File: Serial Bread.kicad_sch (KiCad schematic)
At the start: 20 parts, among them J1 TYPE-C-31-M-12, J2 Conn_02x04_Top_Bottom, U1 CH340C, U2 AP2112K-3.3

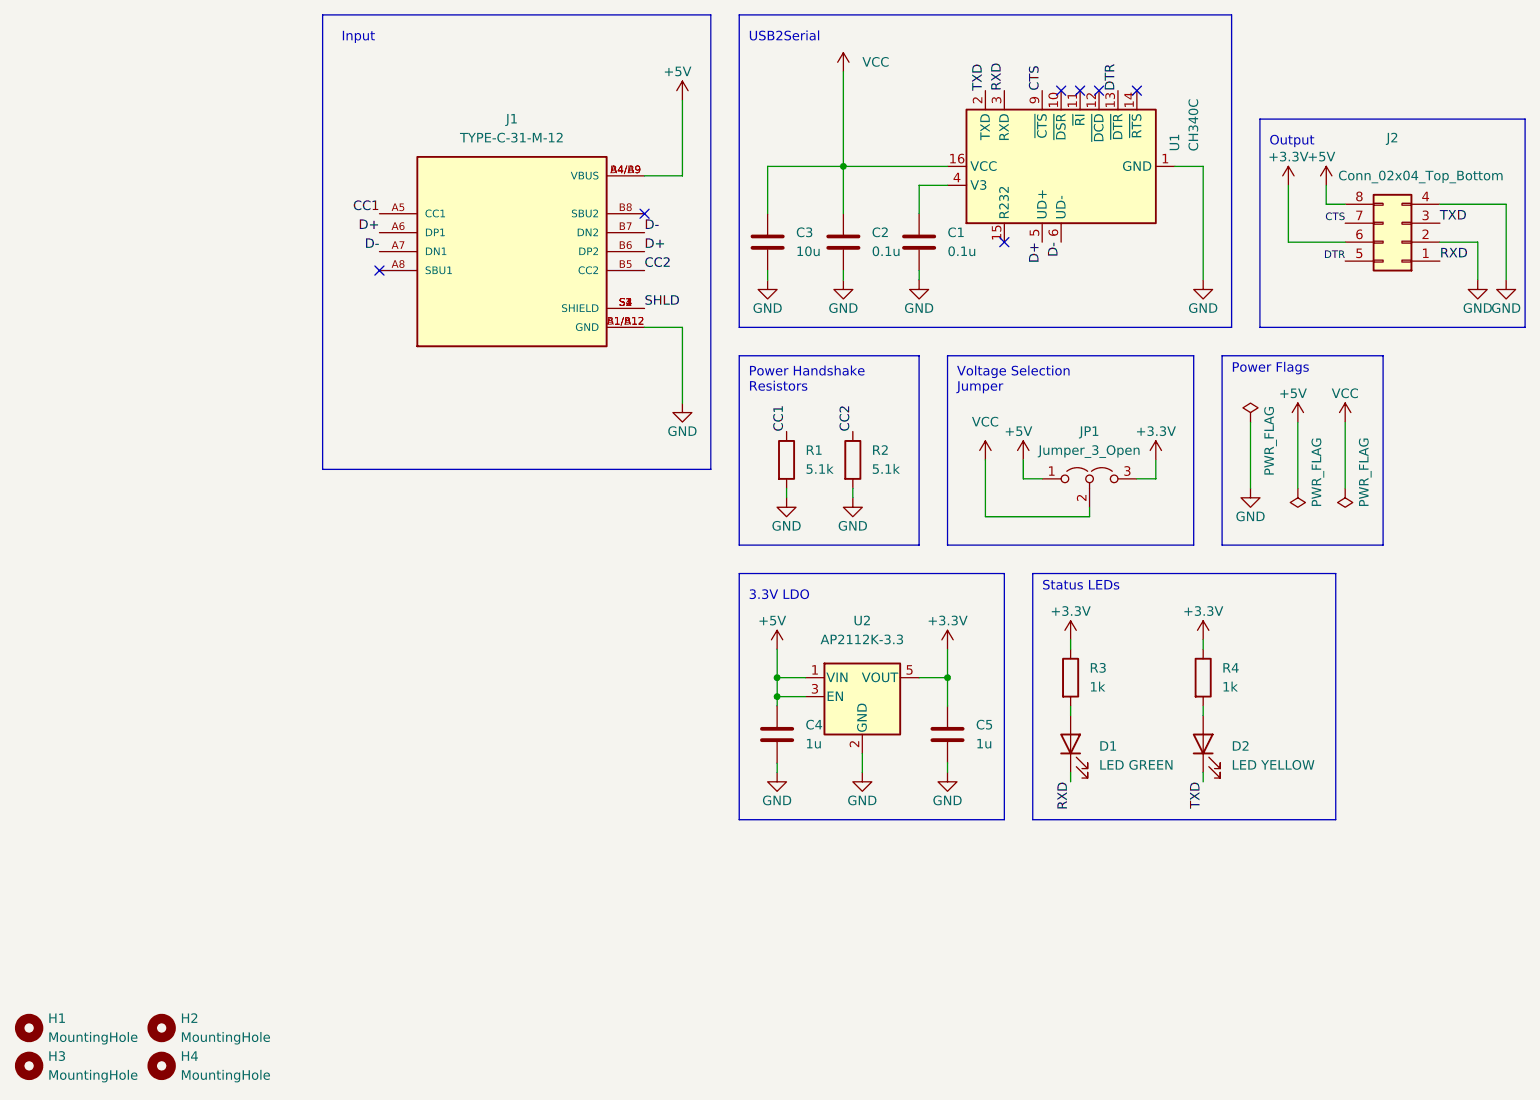
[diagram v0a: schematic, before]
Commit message: Initial commit R1.1
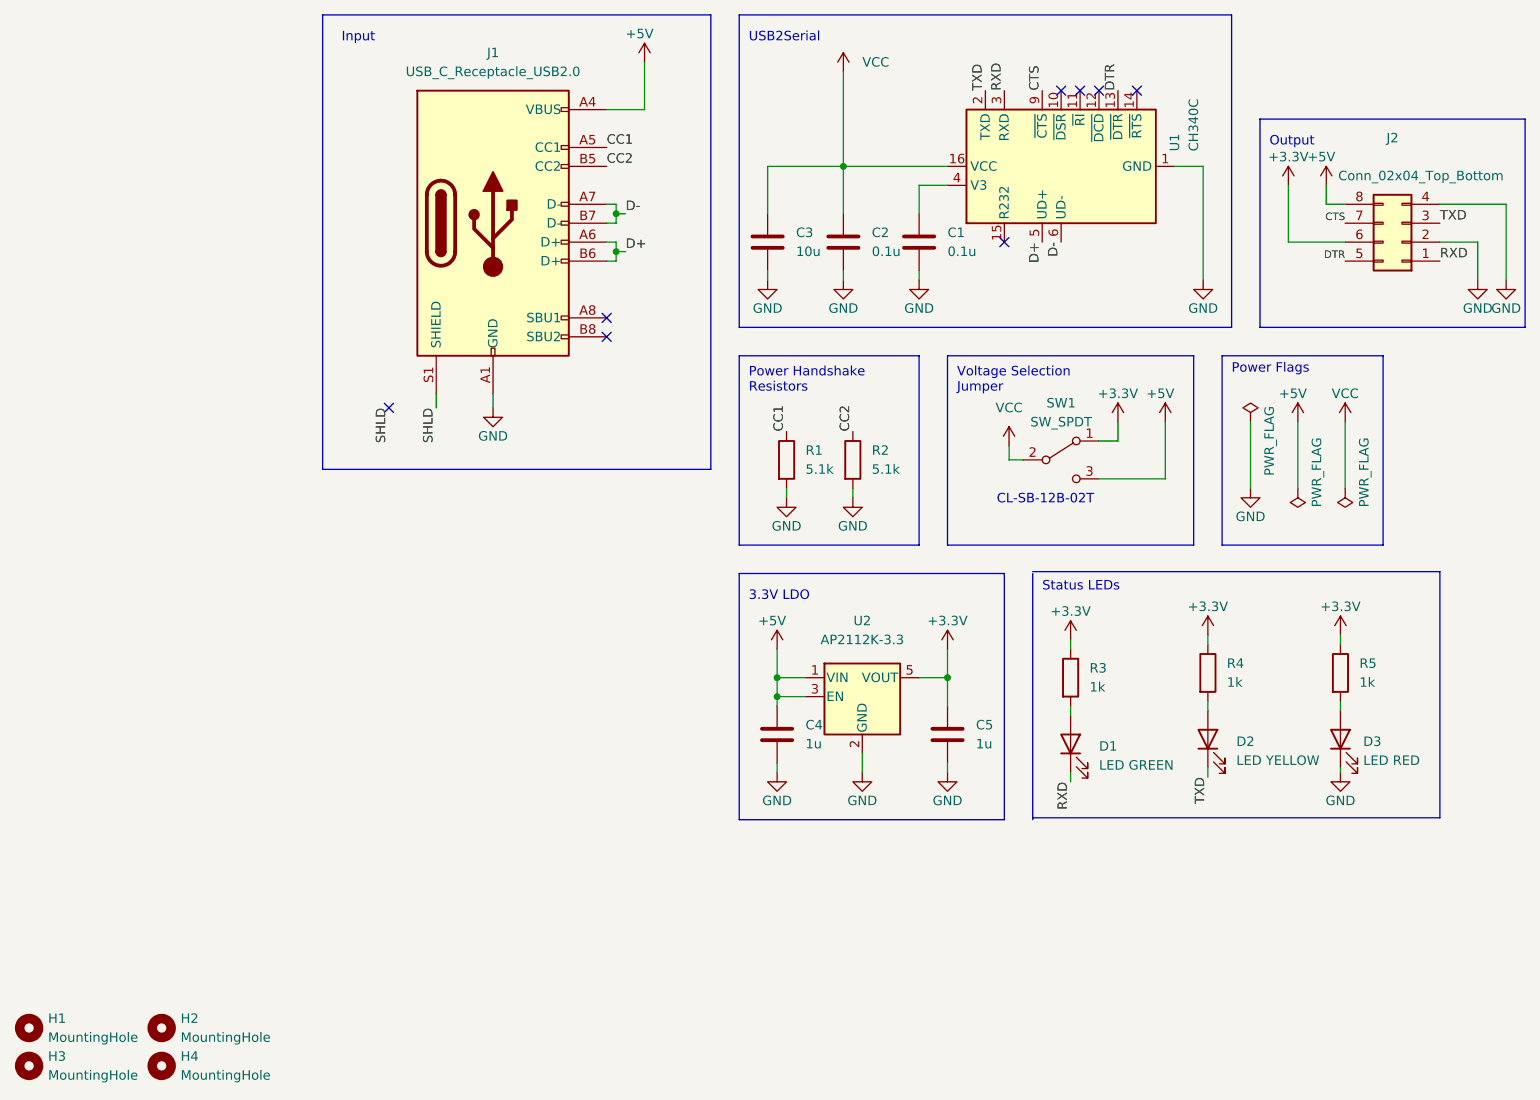
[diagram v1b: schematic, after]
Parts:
- removed J1: TYPE-C-31-M-12, SnapEDA Library:HRO_TYPE-C-31-M-12, symbol TYPE-C-31-M-12:TYPE-C-31-M-12
- removed JP1: Jumper_3_Open, Connector_PinHeader_1.27mm:PinHeader_1x03_P1.27mm_Vertical, symbol Jumper:Jumper_3_Open
- added D3: LED RED, LED_SMD:LED_0603_1608Metric, symbol Device:LED
- added J1: USB_C_Receptacle_USB2.0, Connector_USB:USB_C_Receptacle_HRO_TYPE-C-31-M-12, symbol Connector:USB_C_Receptacle_USB2.0
- added R5: 1k, Resistor_SMD:R_0402_1005Metric, symbol Device:R
- added SW1: SW_SPDT, Custom_Switches:CL-SB-12B-02T, symbol Switch:SW_SPDT
- C1, C2: footprint Capacitor_SMD:C_0603_1608Metric -> Capacitor_SMD:C_0402_1005Metric; MPN C14663 -> C1525
- C3: footprint Capacitor_SMD:C_0603_1608Metric -> Capacitor_SMD:C_0402_1005Metric; MPN C19702 -> C15525
- C4, C5: footprint Capacitor_SMD:C_0603_1608Metric -> Capacitor_SMD:C_0402_1005Metric; MPN C15849 -> C52923
- J2: MPN C2833740 -> C358726
- R1, R2: footprint Resistor_SMD:R_0603_1608Metric -> Resistor_SMD:R_0402_1005Metric; MPN C23186 -> C25905
- R3, R4: footprint Resistor_SMD:R_0603_1608Metric -> Resistor_SMD:R_0402_1005Metric; MPN C21190 -> C11702
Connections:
- net +3.3V: now also R5.1, SW1.1 (A)
- net +5V: now also J1.A4 (VBUS), J1.A9 (VBUS), J1.B4 (VBUS), J1.B9 (VBUS), SW1.3 (C)
- net CC1: now also J1.A5 (CC1)
- net CC2: now also J1.B5 (CC2)
- net D+: now also J1.A6 (D+), J1.B6 (D+)
- net D-: now also J1.A7 (D-), J1.B7 (D-)
- net GND: now also D3.1 (K), J1.A1 (GND), J1.A12 (GND), J1.B1 (GND), J1.B12 (GND)
- net SHLD: now also J1.S1 (SHIELD)
- net VCC: now also SW1.2 (B)
- new net: D3.2 (A), R5.2
- no-connect marks 7 -> 8
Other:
- note added: "CL-SB-12B-02T"
- moved on the sheet: D2, R4
